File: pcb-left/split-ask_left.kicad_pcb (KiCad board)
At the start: 2 copper layers, 165.4 x 98.7 mm, 59 parts, among them J1 MJ-4PP-9, SW1 SW_PUSH, SW10 SW_PUSH, SW11 SW_PUSH, SW12 SW_PUSH, SW13 SW_PUSH, SW14 SW_PUSH, SW15 SW_PUSH, SW16 SW_PUSH, SW17 SW_PUSH, SW18 SW_PUSH, SW19 SW_PUSH, SW2 SW_PUSH, SW20 SW_PUSH, SW21 SW_PUSH, SW22 SW_PUSH, SW23 SW_PUSH, SW24 SW_PUSH, SW25 SW_PUSH, SW26 SW_PUSH, SW27 SW_PUSH, SW28 SW_PUSH, SW3 SW_PUSH, SW4 SW_PUSH, SW5 SW_PUSH, SW6 SW_PUSH, SW7 SW_PUSH, SW8 SW_PUSH, SW9 SW_PUSH, U1 ProMicro

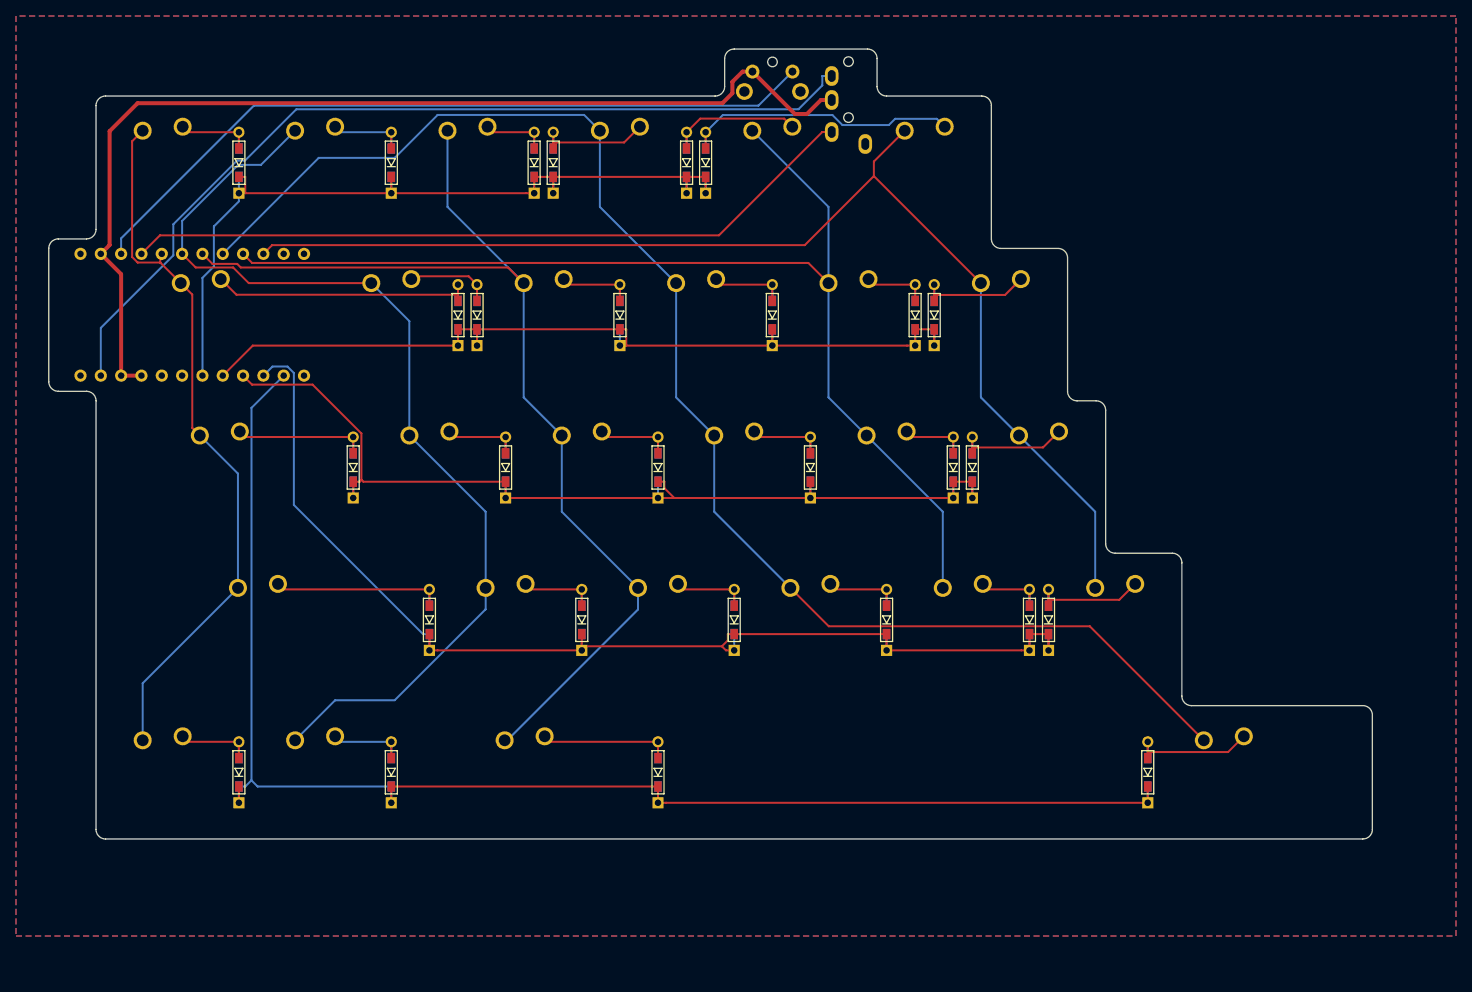
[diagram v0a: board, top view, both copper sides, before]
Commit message: update
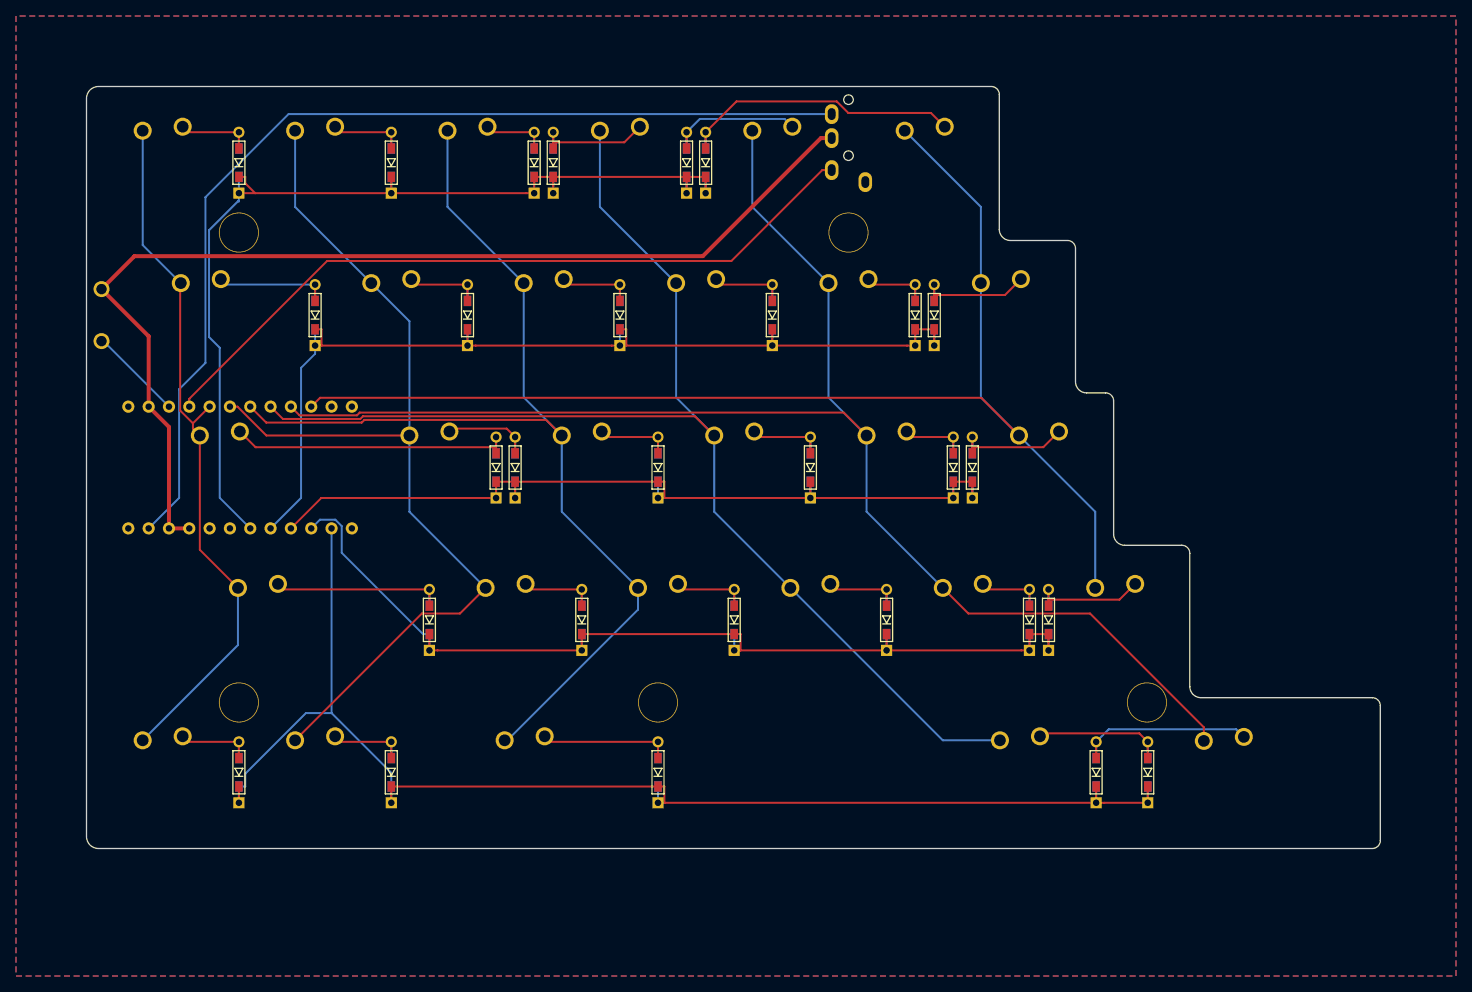
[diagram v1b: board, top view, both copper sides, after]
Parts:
- added D29: D, kbd:D3_TH_SMD, F.Cu at (150.0, 109.5)
- added HOLE1: HOLE, kbd:HOLE, F.Cu at (42.9, 42.1)
- added HOLE2: Val**, kbd:HOLE, F.Cu at (119.1, 42.1)
- added HOLE3: HOLE, kbd:HOLE, F.Cu at (42.9, 100.8)
- added HOLE4: HOLE, kbd:HOLE, F.Cu at (95.2, 100.8)
- added HOLE5: HOLE, kbd:HOLE, F.Cu at (156.4, 100.8)
- added SW29: SW_PUSH, Alps_Only:ALPS-1U, F.Cu at (166.0, 109.6)
- RST1: footprint Keebio-Parts:SW_Tactile_SPST_Angled_MJTP1117 -> kbd:ResetSW_1side
- moved RST1 91.6 mm to (25.7, 52.4), turned to 270 degrees
- moved SW28 25.5 mm to (140.5, 109.5)
- moved U1 20.0 mm to (43.5, 71.4)
- moved D13 17.9 mm to (75.0, 71.4)
- moved D7 17.9 mm to (52.4, 52.4)
- moved J1 4.76 mm to (119.1, 24.0)
- moved D14 1.19 mm to (77.4, 71.4)
- moved D8 1.19 mm to (71.4, 52.4)
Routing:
- net reset: track 94.5 -> 11.8 mm
- net col4: track 141.7 -> 182.3 mm
- net Net-(D29-Pad2): track 0.00 -> 23.6 mm
- net col3: track 181.7 -> 158.3 mm
- net row3: track 147.6 -> 125.9 mm
- net row0: track 108.3 -> 129.7 mm
- net Net-(D13-Pad2): track 18.5 -> 36.9 mm
- net Net-(D7-Pad2): track 34.5 -> 16.1 mm
- net row4: track 183.2 -> 167.6 mm
- net row2: track 126.9 -> 112.0 mm
- net data: track 113.3 -> 126.9 mm
- net row1: track 115.7 -> 128.6 mm
- net col5: track 150.5 -> 157.9 mm
- net GND: track 131.7 -> 135.0 mm
- net col1: track 125.4 -> 122.6 mm
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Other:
- board size 165.4 x 98.7 mm -> 161.7 x 95.2 mm
- board text added: "Split ASK: Left Side / PCB Designed by Ryo Nakae"
